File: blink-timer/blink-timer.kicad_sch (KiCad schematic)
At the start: 14 parts, among them J1 Conn_01x04_Socket, Q1 IRF4905, U1 LM393

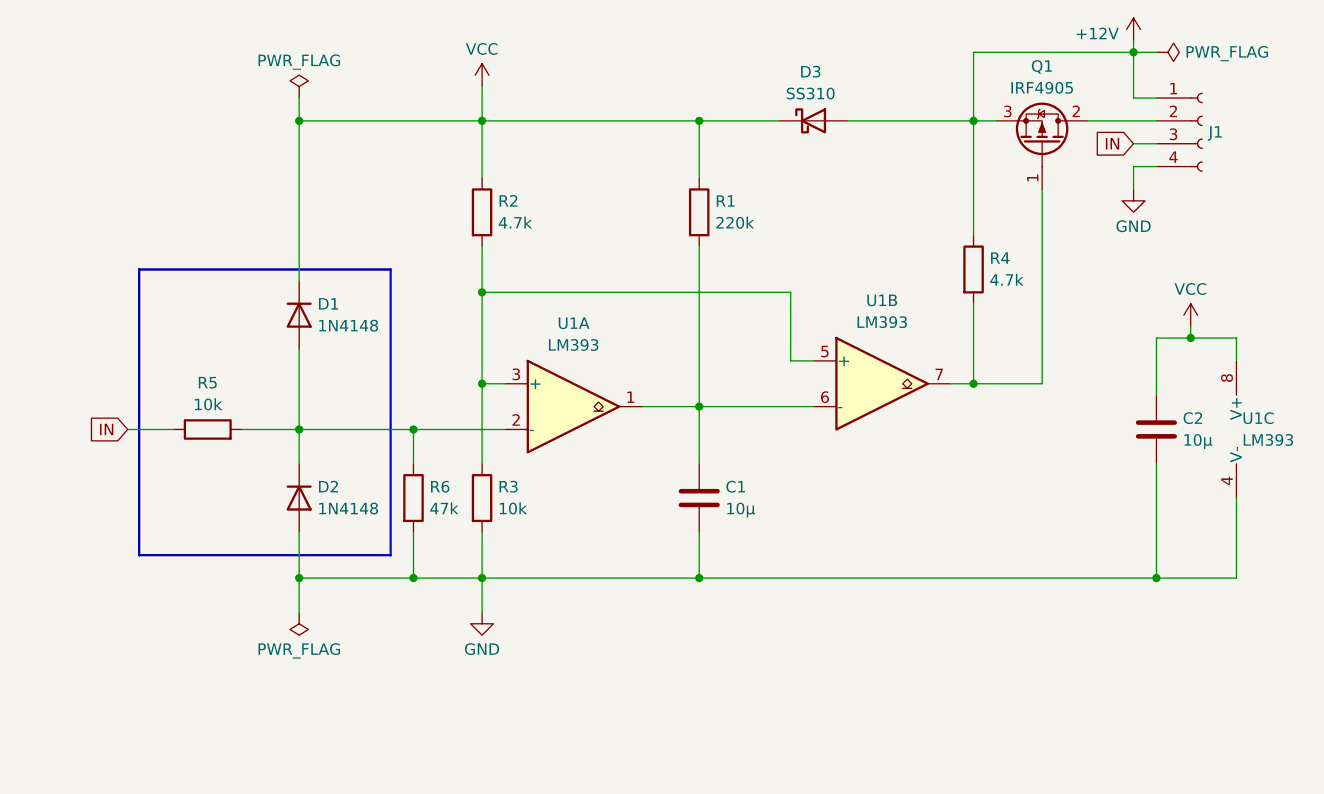
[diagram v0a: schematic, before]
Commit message: tunk
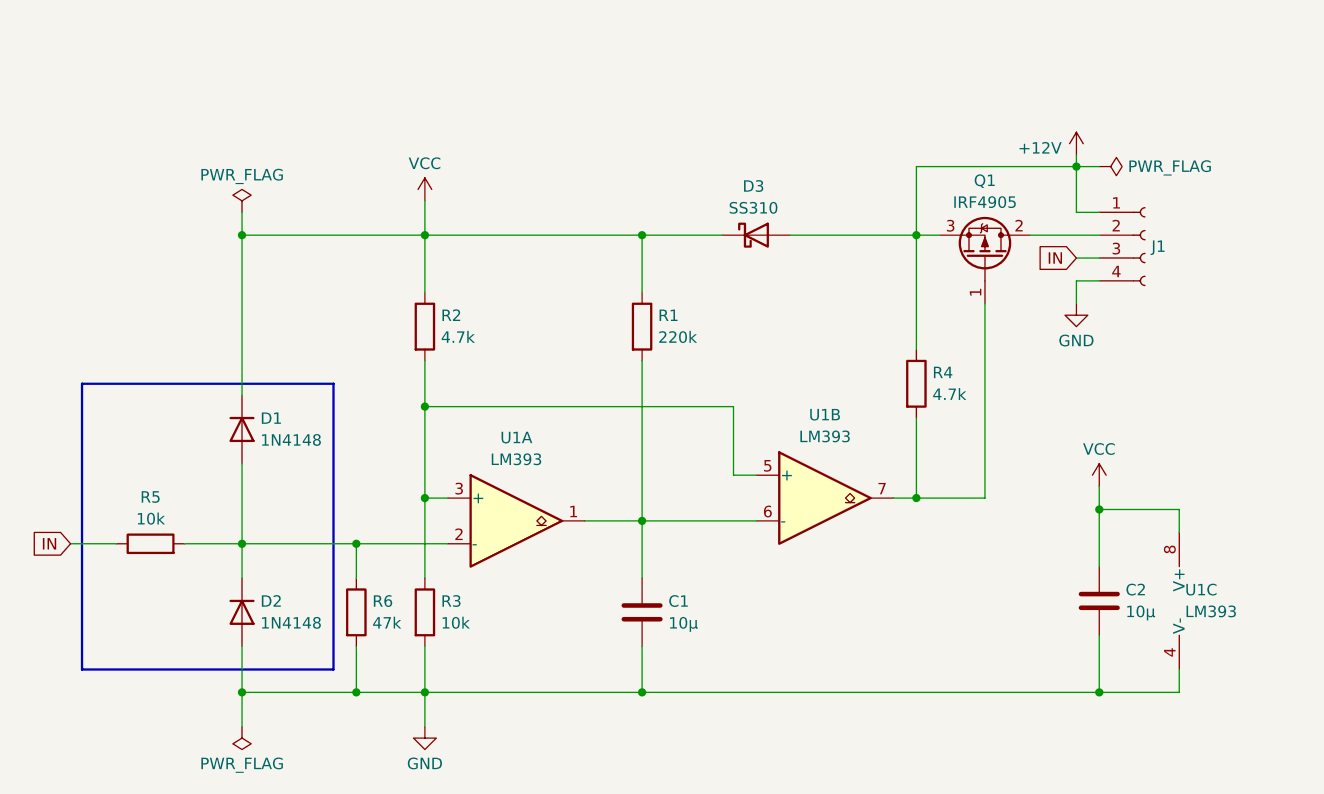
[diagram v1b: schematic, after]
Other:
- moved on the sheet: C1, C2, D1, D2, D3, J1, Q1, R1, R2, R3, R4, R5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
